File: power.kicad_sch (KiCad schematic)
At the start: 17 parts, among them J2 USB_C_Receptacle_USB2.0, SW2 SW_SPDT, U3 BQ24075, U4 XC6206B331MR, U5 LN4913, U8 SRV05-4

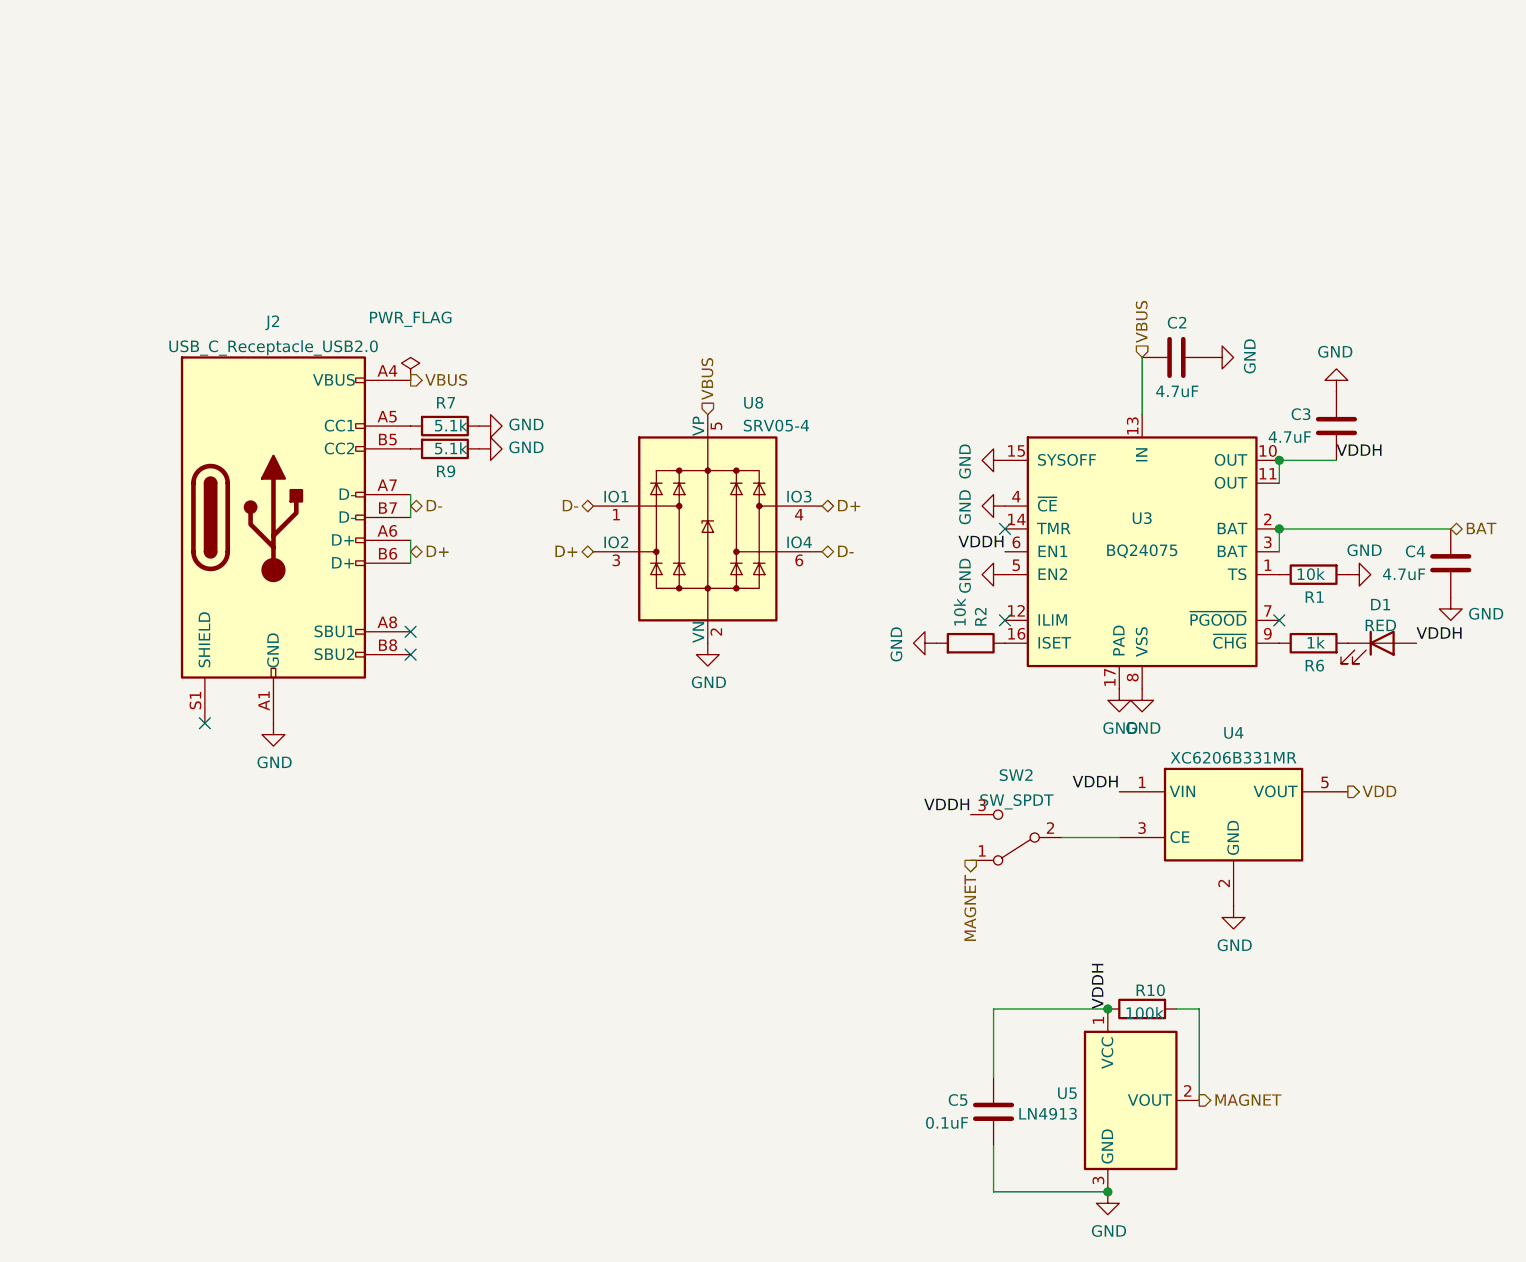
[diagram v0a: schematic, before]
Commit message: backup & remove useless things
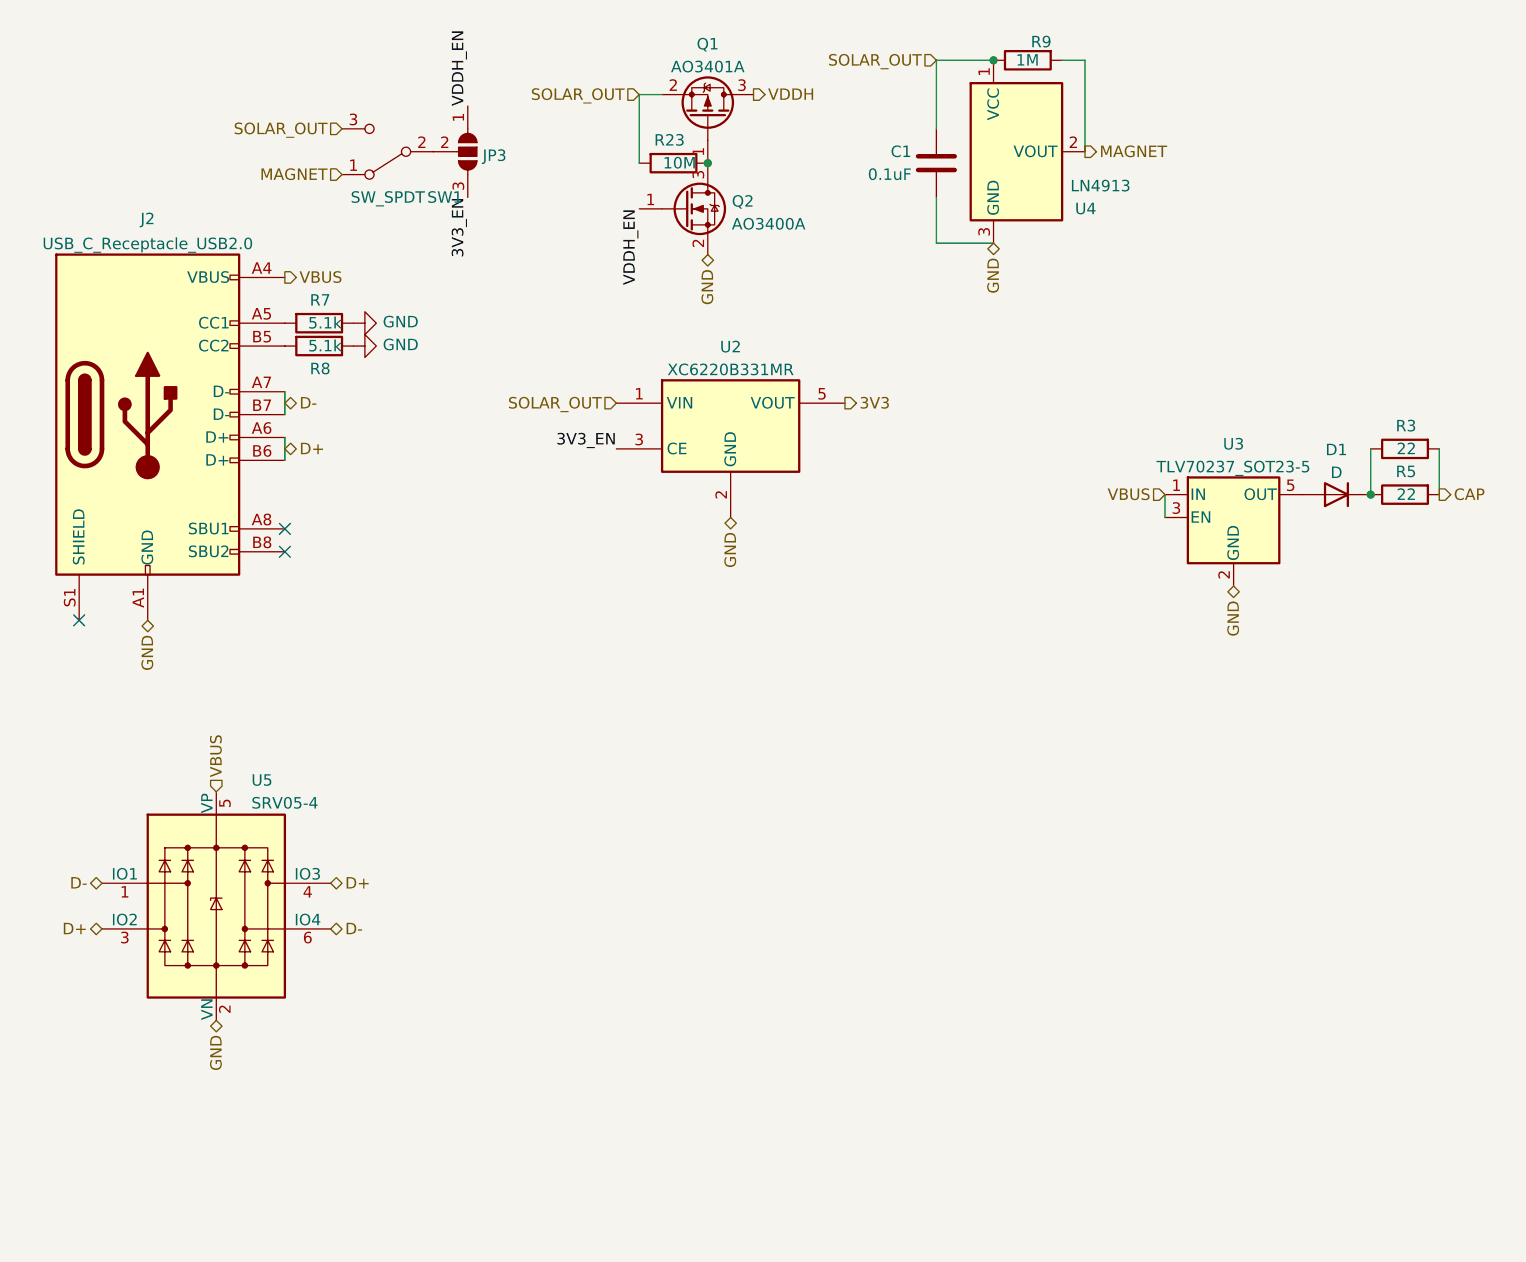
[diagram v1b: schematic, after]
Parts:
- removed C2, C3, C4: 4.7uF, Capacitor_SMD:C_0603_1608Metric, symbol Device:C
- removed D1: RED, LED_SMD:LED_0805_2012Metric, symbol Device:LED
- removed R1, R2: 10k, Resistor_SMD:R_0603_1608Metric, symbol Device:R
- removed R6: 1k, Resistor_SMD:R_0603_1608Metric, symbol Device:R
- removed U3: BQ24075, Package_DFN_QFN:VQFN-16-1EP_3x3mm_P0.5mm_EP1.68x1.68mm_ThermalVias, symbol Battery_Management:BQ24075
- removed U4: XC6206B331MR, Package_TO_SOT_SMD:SOT-23-5, symbol Regulator_Linear:XC6220B331MR
- added D1: D, Diode_SMD:D_SOD-123, symbol Device:D
- added JP3: SolderJumper_3_Open, Jumper:SolderJumper-3_P1.3mm_Open_RoundedPad1.0x1.5mm, symbol Jumper:SolderJumper_3_Open
- added Q1: AO3401A, Package_TO_SOT_SMD:SOT-23, symbol Transistor_FET:AO3401A
- added Q2: AO3400A, Package_TO_SOT_SMD:SOT-23, symbol Transistor_FET:AO3400A
- added R23: 10M, Resistor_SMD:R_0603_1608Metric, symbol Device:R
- added R3, R5: 22, Resistor_SMD:R_0603_1608Metric, symbol Device:R
- added U2: XC6220B331MR, Package_TO_SOT_SMD:SOT-23-5, symbol Regulator_Linear:XC6220B331MR
- added U3: TLV70237_SOT23-5, Package_TO_SOT_SMD:SOT-23-5, symbol Regulator_Linear:TLV70237_SOT23-5
- R9: renamed from R10; value 100k -> 1M
- renumbered C5 to C1, R9 to R8, SW2 to SW1, U5 to U4, U8 to U5
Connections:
- net GND: now also Q2.2 (S), U2.2 (GND), U3.2 (GND)
- net VBUS: now also U3.1 (IN), U3.3 (EN)
- net VDDH: now also Q1.3 (D); no longer C1.1, R9.1, SW1.3 (C), U4.1 (VCC)
- net at SW1.2 (B): now also JP3.2 (C)
- new net: Q1.1 (G), Q2.3 (D), R23.1
- new net: D1.1 (K), R3.1, R5.1
- new net: D1.2 (A), U3.5 (OUT)
- new net 3V3: U2.5 (VOUT)
- new net 3V3_EN: JP3.3 (B), U2.3 (CE)
- new net CAP: R3.2, R5.2
- new net SOLAR_OUT: C1.1, Q1.2 (S), R23.2, R9.1, SW1.3 (C), U2.1 (VIN), U4.1 (VCC)
- new net VDDH_EN: JP3.1 (A), Q2.1 (G)
- no-connect marks 6 -> 3
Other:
- moved on the sheet: C1, J2, R7, R8, R9, SW1, U4, U5
